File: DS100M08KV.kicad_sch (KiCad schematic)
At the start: 128 parts, among them J1 wire2board, J10 BNC_panel_mount, J11 wire2board, J2 Wire2Board, J3 wire2board, J4 wire2board, J5 Wire2Board, J6 Wire2Board, J7 Wire2Board, J8 red_safety_4mm_connector, J9 black_safety_4mm_connector, Q1 BD679, Q2 FS8205A, Q4 BD680, SW1 SW_DPDT_x2, SW2 SW_DPDT_x2, U1 AD8039, U2 TP4056, U4 AD8009, U5 DW01A, U7 TLV61070ADBVR

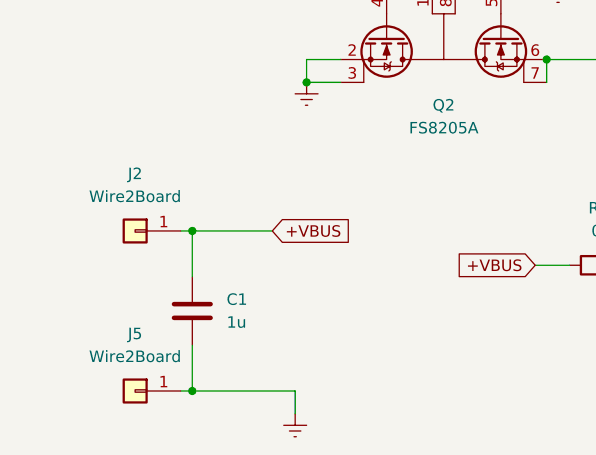
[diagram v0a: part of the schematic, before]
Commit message: Clearer
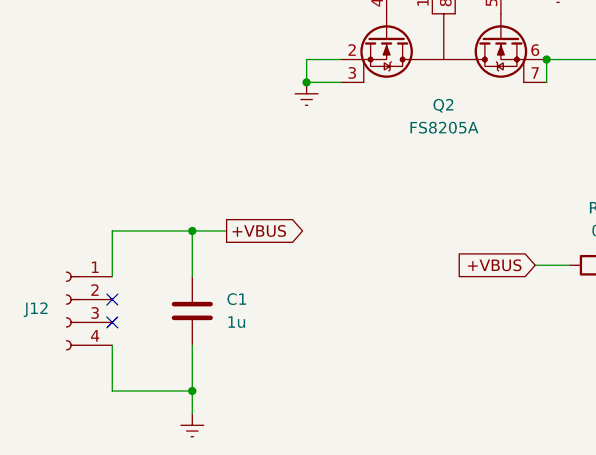
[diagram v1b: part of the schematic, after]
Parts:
- removed J2, J5: Wire2Board, Connector_Wire:SolderWire-0.127sqmm_1x01_D0.48mm_OD1mm, symbol Connectors_and_wire_to_board:Wire2Board
- added J12: Conn_01x04_Socket, Connector_JST:JST_PH_B4B-PH-K_1x04_P2.00mm_Vertical, symbol Connector:Conn_01x04_Socket
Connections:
- net +VBUS: now also J12.1 (Pin_1)
- net Earth: now also J12.4 (Pin_4)
- no-connect marks 2 -> 4
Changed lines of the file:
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@@
 	)
 	(no_connect
+		(at 26.67 247.65)
+	)
+	(no_connect
+		(at 26.67 250.19)
+	)
+	(no_connect
 		(at 90.17 256.54)
 	)
 	(wire
 		(pts
-			(xy 34.29 257.81) (xy 35.56 257.81)
+			(xy 26.67 257.81) (xy 35.56 257.81)
 		)
 		(stroke
@@
 	(wire
 		(pts
-			(xy 46.99 257.81) (xy 46.99 260.35)
+			(xy 35.56 257.81) (xy 35.56 260.35)
+		)
+		(stroke
+			(width 0)
+			(type default)
+		)
+	)
+	(wire
+		(pts
+			(xy 26.67 245.11) (xy 26.67 240.03)
 		)
 		(stroke
@@
 	(wire
 		(pts
+			(xy 26.67 252.73) (xy 26.67 257.81)
+		)
+		(stroke
+			(width 0)
+			(type default)
+		)
+	)
+	(wire
+		(pts
 			(xy 367.03 107.95) (xy 378.46 107.95)
 		)
@@
 	(wire
 		(pts
+			(xy 26.67 240.03) (xy 35.56 240.03)
+		)
+		(stroke
+			(width 0)
+			(type default)
+		)
+	)
+	(wire
+		(pts
 			(xy 328.93 85.09) (xy 335.28 85.09)
 		)
@@
 	(wire
 		(pts
-			(xy 35.56 257.81) (xy 46.99 257.81)
-		)
-		(stroke
-			(width 0)
-			(type default)
-		)
-	)
-	(wire
-		(pts
 			(xy 331.47 40.64) (xy 322.58 40.64)
 		)
@@
 	(wire
 		(pts
-			(xy 35.56 240.03) (xy 44.45 240.03)
+			(xy 35.56 240.03) (xy 39.37 240.03)
 		)
 		(stroke
@@
 	(wire
 		(pts
-			(xy 34.29 240.03) (xy 35.56 240.03)
-		)
-		(stroke
-			(width 0)
-			(type default)
-		)
-	)
-	(wire
-		(pts
 			(xy 321.31 85.09) (xy 328.93 85.09)
 		)
@@
 	)
 	(global_label "+VBUS"
-		(shape input)
-		(at 44.45 240.03 0)
+		(shape output)
+		(at 39.37 240.03 0)
 		(fields_autoplaced yes)
 		(effects
@@
 		)
 		(property "Intersheetrefs" "${INTERSHEET_REFS}"
-			(at 53.9062 240.03 0)
+			(at 48.8262 240.03 0)
 			(effects
 				(font
@@
 	(symbol
 		(lib_id "power:Earth")
-		(at 46.99 260.35 0)
+		(at 35.56 260.35 0)
 		(unit 1)
 		(exclude_from_sim no)
@@
 		(fields_autoplaced yes)
 		(property "Reference" "#PWR07"
-			(at 46.99 266.7 0)
+			(at 35.56 266.7 0)
 			(effects
 				(font
@@
 		)
 		(property "Value" "Earth"
-			(at 46.99 265.43 0)
+			(at 35.56 265.43 0)
 			(effects
 				(font
@@
 		)
 		(property "Footprint" ""
-			(at 46.99 260.35 0)
+			(at 35.56 260.35 0)
 			(effects
 				(font
@@
 		)
 		(property "Datasheet" "~"
-			(at 46.99 260.35 0)
+			(at 35.56 260.35 0)
 			(effects
 				(font
@@
 		)
 		(property "Description" "Power symbol creates a global label with name \"Earth\""
-			(at 46.99 260.35 0)
+			(at 35.56 260.35 0)
 			(effects
 				(font
@@
 			)
 		)
-		(property "Description" ""
+		(property "Description" "Switch, dual pole double throw, separate symbols"
 			(at 189.23 180.34 0)
 			(effects
@@
 	)
 	(symbol
-		(lib_id "Connectors_and_wire_to_board:Wire2Board")
-		(at 29.21 240.03 0)
-		(mirror y)
-		(unit 1)
-		(exclude_from_sim no)
-		(in_bom yes)
-		(on_board yes)
-		(dnp no)
-		(fields_autoplaced yes)
-		(property "Reference" "J2"
-			(at 29.21 233.68 0)
-			(effects
-				(font
-					(size 1.27 1.27)
-				)
-			)
-		)
-		(property "Value" "Wire2Board"
-			(at 29.21 236.22 0)
-			(effects
-				(font
-					(size 1.27 1.27)
-				)
-			)
-		)
-		(property "Footprint" "Connector_Wire:SolderWire-0.127sqmm_1x01_D0.48mm_OD1mm"
-			(at 29.21 240.03 0)
-			(effects
-				(font
-					(size 1.27 1.27)
-				)
-				(hide yes)
-			)
-		)
-		(property "Datasheet" "~"
-			(at 29.21 240.03 0)
-			(effects
-				(font
-					(size 1.27 1.27)
-				)
-				(hide yes)
-			)
-		)
-		(property "Description" ""
-			(at 29.21 240.03 0)
-			(effects
-				(font
-					(size 1.27 1.27)
-				)
-				(hide yes)
-			)
-		)
-		(pin "1"
-		)
-		(instances
-			(project "DS100M06V_linear"
-				(path "/e034a6c3-9973-4355-8043-c1e988e27610"
-					(reference "J2")
-					(unit 1)
-				)
-			)
-		)
-	)
-	(symbol
 		(lib_id "Device:R_Potentiometer")
 		(at 163.83 71.12 180)
@@
 	)
 	(symbol
+		(lib_id "Connector:Conn_01x04_Socket")
+		(at 21.59 247.65 0)
+		(mirror y)
+		(unit 1)
+		(exclude_from_sim no)
+		(in_bom yes)
+		(on_board yes)
+		(dnp no)
+		(property "Reference" "J12"
+			(at 18.288 248.666 0)
+			(effects
+				(font
+					(size 1.27 1.27)
+				)
+			)
+		)
+		(property "Value" "Conn_01x04_Socket"
+			(at 22.225 242.57 0)
+			(effects
+				(font
+					(size 1.27 1.27)
+				)
+				(hide yes)
+			)
+		)
+		(property "Footprint" "Connector_JST:JST_PH_B4B-PH-K_1x04_P2.00mm_Vertical"
+			(at 21.59 247.65 0)
+			(effects
+				(font
+					(size 1.27 1.27)
+				)
+				(hide yes)
+			)
+		)
+		(property "Datasheet" "~"
+			(at 21.59 247.65 0)
+			(effects
+				(font
+					(size 1.27 1.27)
+				)
+				(hide yes)
+			)
+		)
+		(property "Description" "Generic connector, single row, 01x04, script generated"
+			(at 21.59 247.65 0)
+			(effects
+				(font
+					(size 1.27 1.27)
+				)
+				(hide yes)
+			)
+		)
+		(pin "3"
+		)
+		(pin "4"
+		)
+		(pin "2"
+		)
+		(pin "1"
+		)
+		(instances
+			(project ""
+				(path "/e034a6c3-9973-4355-8043-c1e988e27610"
+					(reference "J12")
+					(unit 1)
+				)
+			)
+		)
+	)
+	(symbol
 		(lib_id "Simulation_SPICE:0")
 		(at 369.57 74.93 0)
@@
 					(unit 1)
 				)
-			)
-		)
-	)
-	(symbol
-		(lib_id "Connectors_and_wire_to_board:Wire2Board")
-		(at 29.21 257.81 0)
-		(mirror y)
-		(unit 1)
-		(exclude_from_sim no)
-		(in_bom yes)
-		(on_board yes)
-		(dnp no)
-		(fields_autoplaced yes)
-		(property "Reference" "J5"
-			(at 29.21 251.46 0)
-			(effects
-				(font
-					(size 1.27 1.27)
-				)
-			)
-		)
-		(property "Value" "Wire2Board"
-			(at 29.21 254 0)
-			(effects
-				(font
-					(size 1.27 1.27)
-				)
-			)
-		)
-		(property "Footprint" "Connector_Wire:SolderWire-0.127sqmm_1x01_D0.48mm_OD1mm"
-			(at 29.21 257.81 0)
-			(effects
-				(font
-					(size 1.27 1.27)
-				)
-				(hide yes)
-			)
-		)
-		(property "Datasheet" "~"
-			(at 29.21 257.81 0)
-			(effects
-				(font
-					(size 1.27 1.27)
-				)
-				(hide yes)
-			)
-		)
-		(property "Description" ""
-			(at 29.21 257.81 0)
-			(effects
-				(font
-					(size 1.27 1.27)
-				)
-				(hide yes)
-			)
-		)
-		(pin "1"
-		)
-		(instances
-			(project "DS100M06V_linear"
-				(path "/e034a6c3-9973-4355-8043-c1e988e27610"
-					(reference "J5")
-					(unit 1)
-				)
